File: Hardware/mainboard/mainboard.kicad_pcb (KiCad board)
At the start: 4 copper layers, 78 x 69.1 mm, 50 parts, among them J1 559592430, J2 status bot, J3 status eot, J4 B02B-XASK-1LFSN, J5 race start, J6 usb-ttl, J7 jtag, J8 KUSBX-SMT-CS-6-BTR, SW1 ON-BOARD, SW2 BOT, SW3 BOOT, U1 S16B-PHDSSLFSN, U2 AMS1117-3.3, U3 STM32F091RCTx, Y1 Crystal_GND24

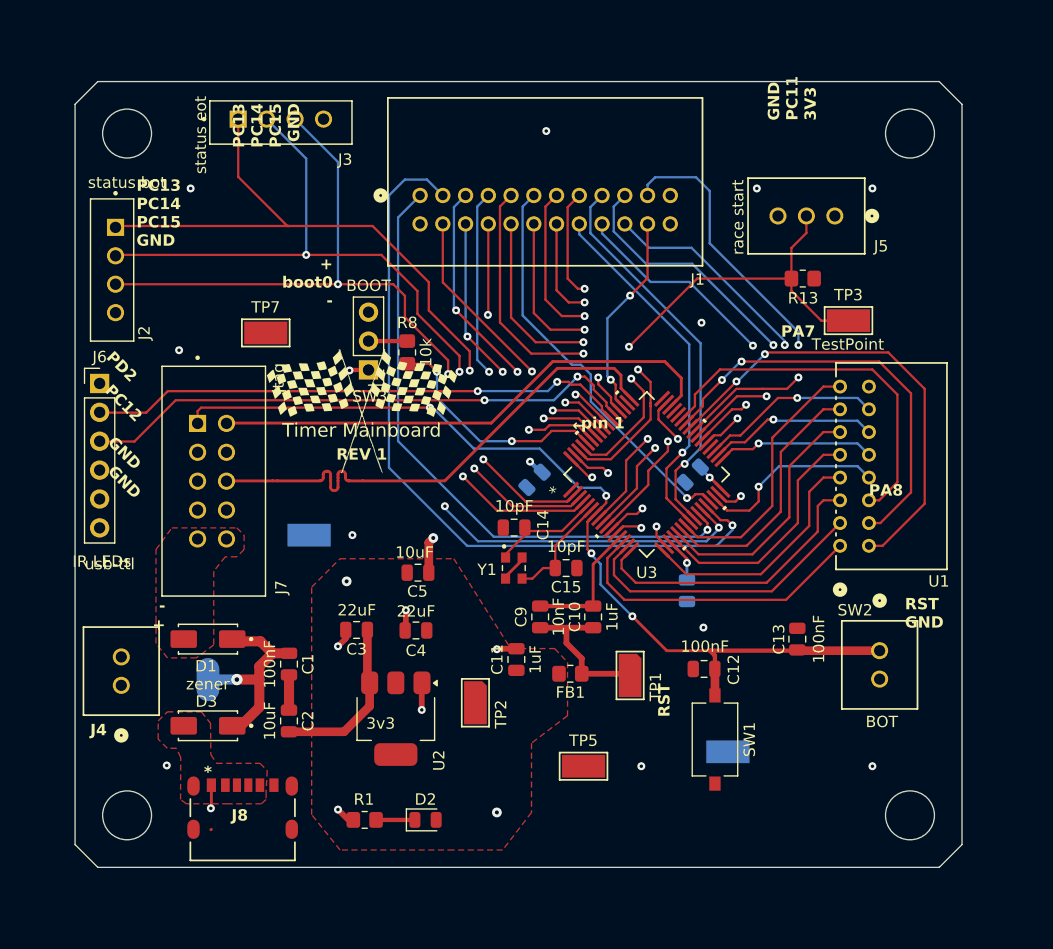
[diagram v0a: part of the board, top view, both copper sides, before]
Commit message: gbr files
ordered pcbs
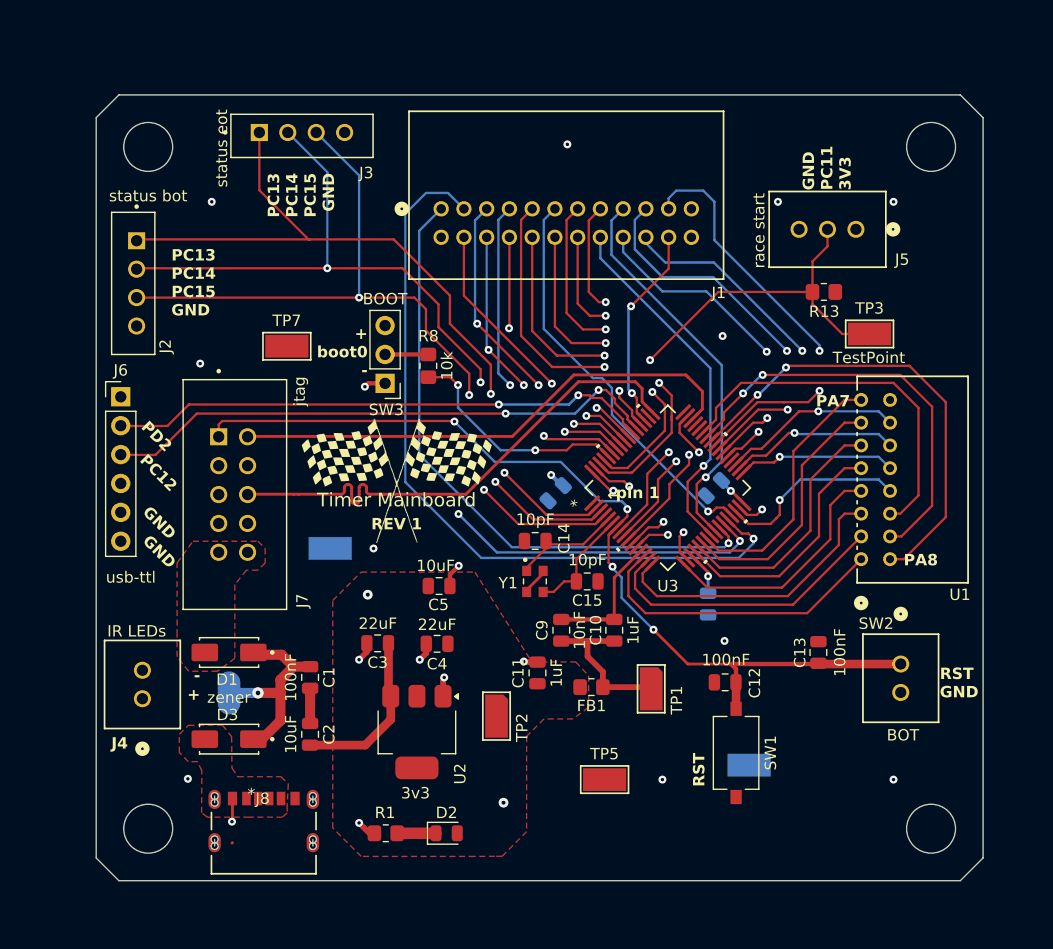
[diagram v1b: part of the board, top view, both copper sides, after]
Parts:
- J8: footprint BIG LIBRARY:usb-c2 -> usbc attempt 3:2171750001_MOL
- moved G*** 6.85 mm to (91.4, 61.1)
- moved R1 2.20 mm to (90.5, 92.1)
- moved SW2 2.20 mm to (135.8, 77.2)
- moved TP8 2.20 mm to (122.4, 86.1)
- moved U1 2.20 mm to (132.3, 68.0)
- moved J1 2.20 mm to (95.4, 37.2)
- moved U3 2.20 mm to (115.3, 61.8)
- moved H2 2.20 mm to (138.4, 31.8)
- moved C3 2.20 mm to (89.8, 75.4)
- moved C4 2.20 mm to (95.0, 75.5)
- moved D1 2.20 mm to (76.7, 76.2)
- moved D3 2.20 mm to (76.7, 83.9)
- moved H4 2.20 mm to (138.4, 91.7)
- moved J2 2.20 mm to (68.6, 43.8)
- moved J5 2.20 mm to (131.8, 39.0)
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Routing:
- net PC9: track 37.9 -> 37.2 mm
- net PB2: track 66.9 -> 67.4 mm
- net /stm/BOOT0: track 20.8 -> 20.3 mm
- net GND: track 30.9 -> 30.4 mm
